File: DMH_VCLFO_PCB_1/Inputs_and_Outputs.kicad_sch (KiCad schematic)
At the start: 7 parts, among them J1 TS_Jack_6.35mm_Sw, J2 TS_Jack_6.35mm_Sw, J200 IDC_02x05, J3 TS_Jack_6.35mm_Sw, J5 TS_Jack_6.35mm_Sw, J50 Conn_01x06, J60 Conn_01x06

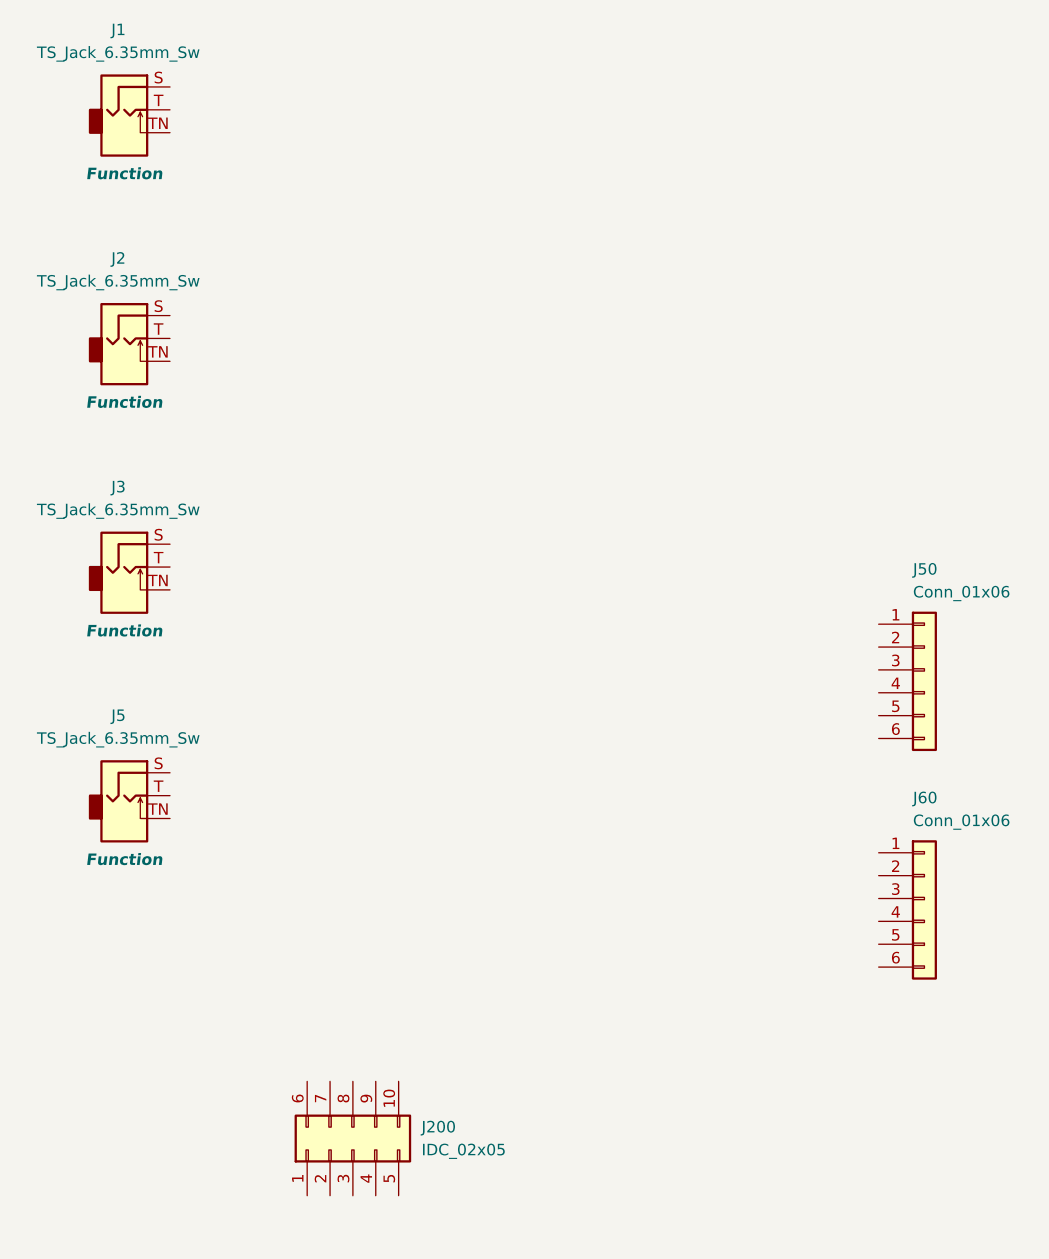
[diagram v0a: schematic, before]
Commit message: schematic design in progress
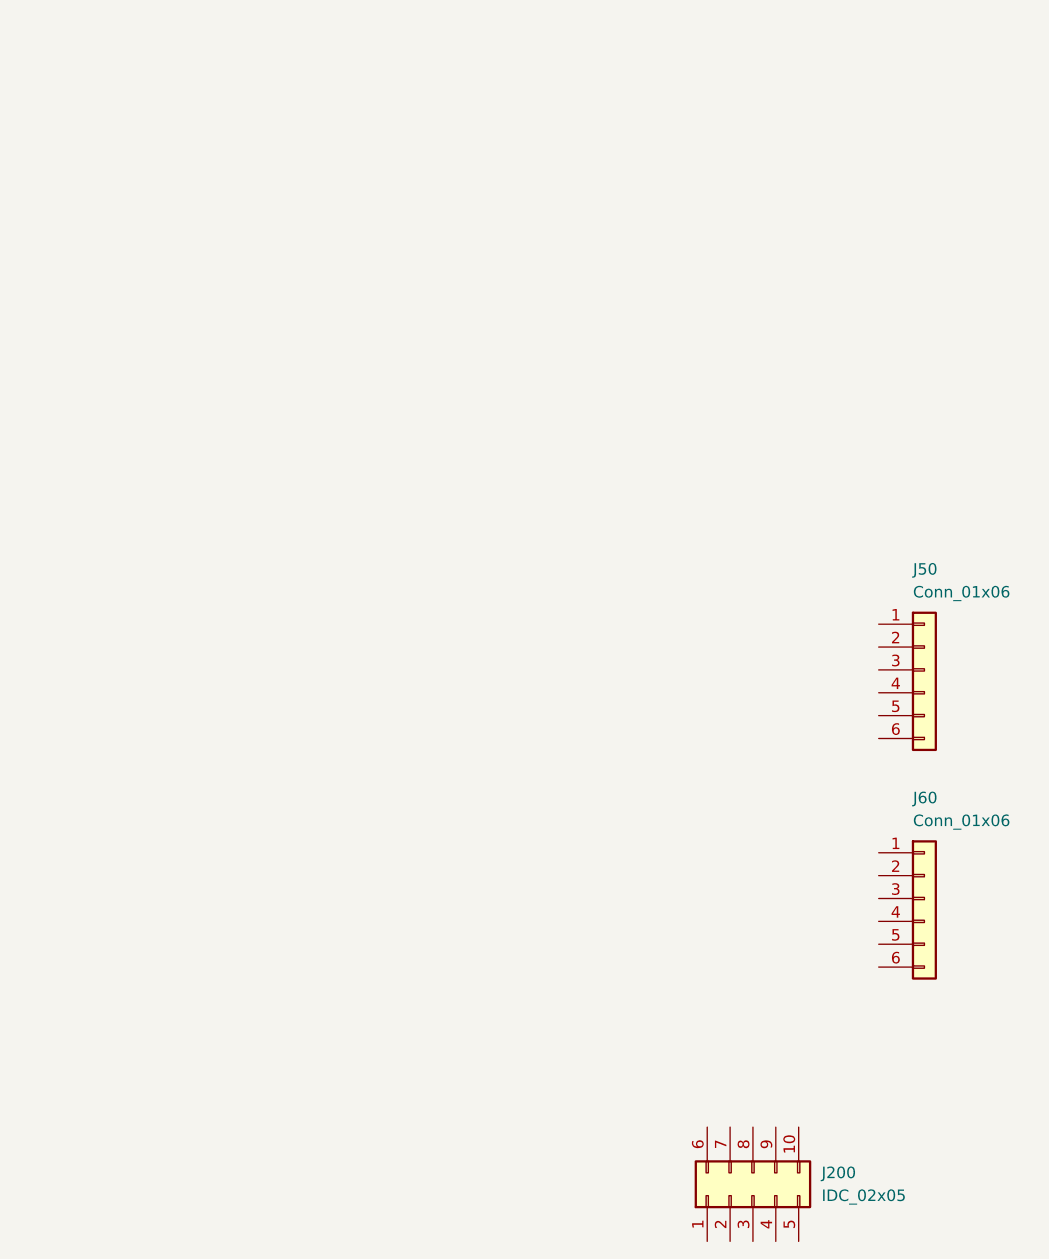
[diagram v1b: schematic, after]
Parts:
- removed J1, J2, J3, J5: TS_Jack_6.35mm_Sw, SynthStuff:CUI_MJ-63052A, symbol SynthStuff:TS_Jack_6.35mm_Sw
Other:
- moved on the sheet: J200

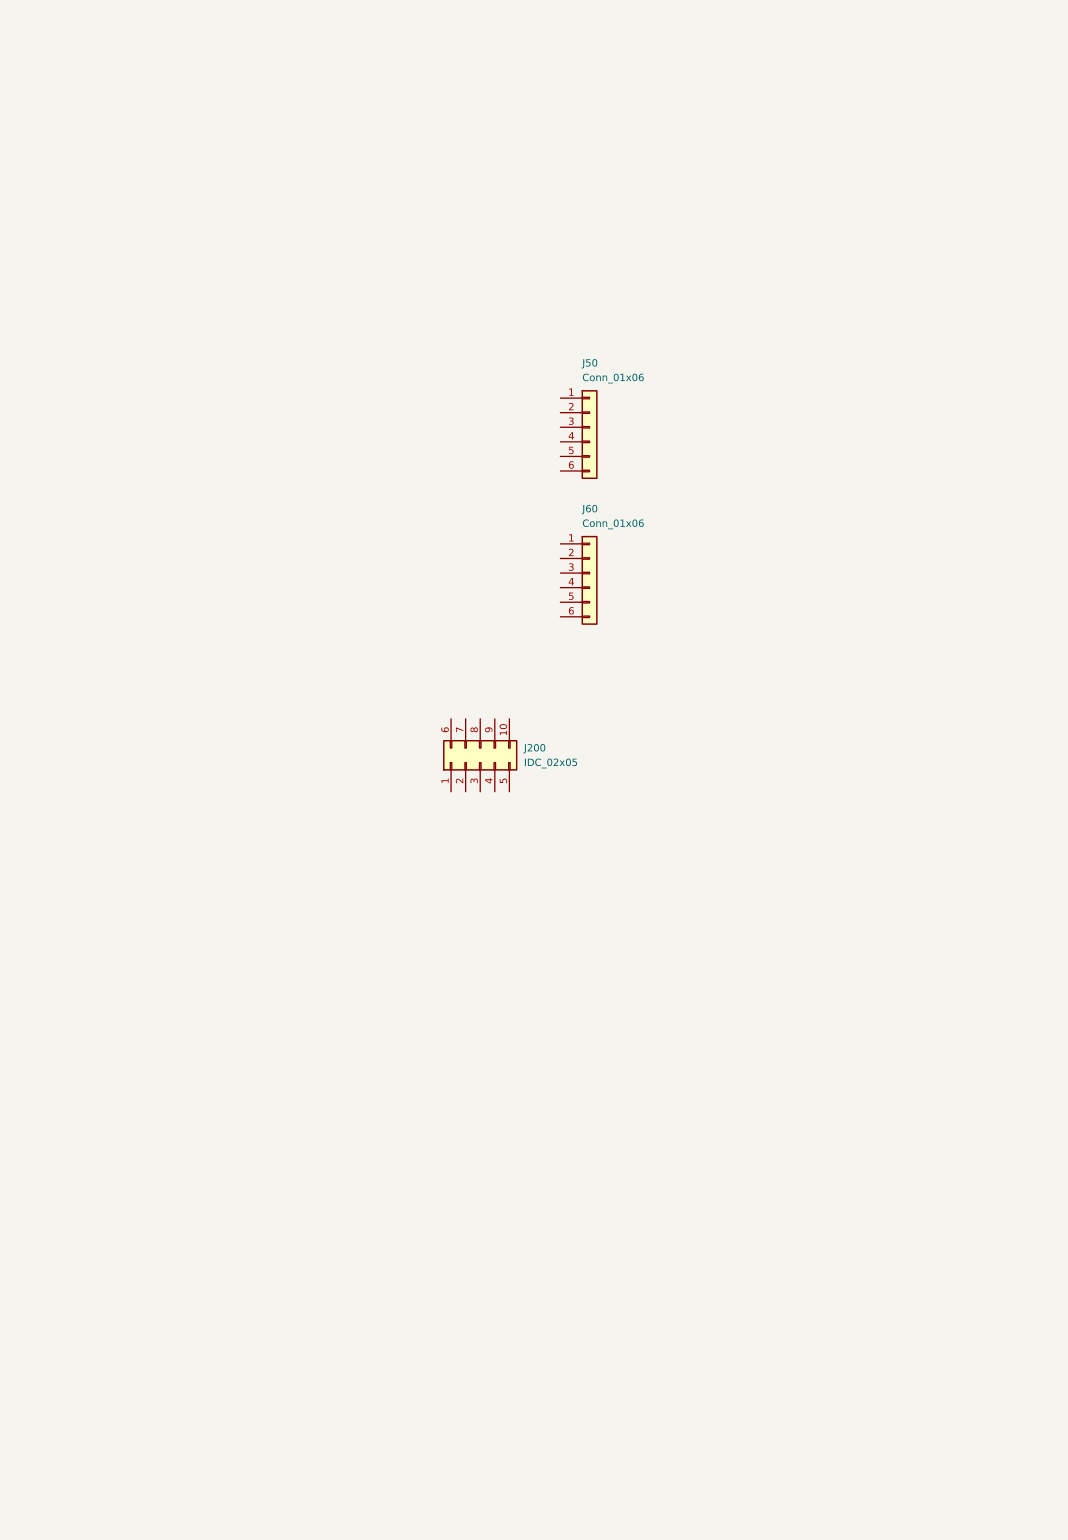
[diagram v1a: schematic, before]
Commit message: Ready for breadboarding
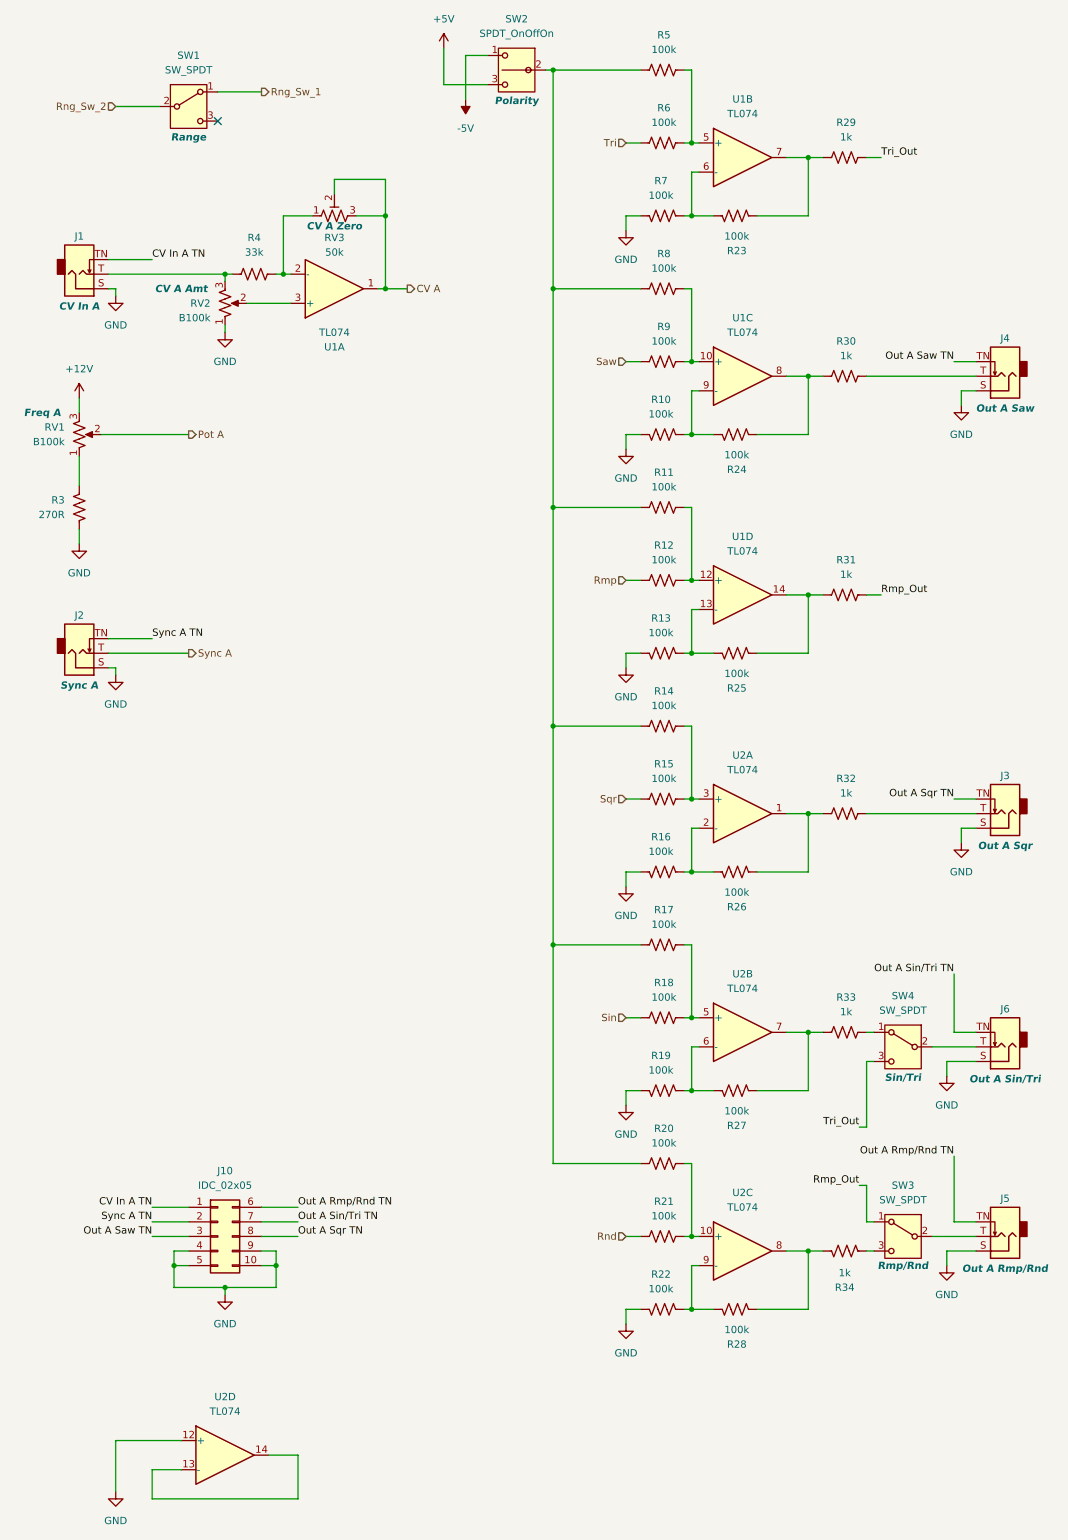
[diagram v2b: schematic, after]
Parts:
- removed J200: IDC_02x05, SynthStuff:IDC-Header_2x05_P2.54mm_Vertical_BackBone, symbol SynthStuff:BackBone_Connector_10Pin
- removed J50, J60: Conn_01x06, Connector_PinSocket_2.54mm:PinSocket_1x06_P2.54mm_Vertical, symbol Connector_Generic:Conn_01x06
- added J1, J2, J3, J4, J5, J6: TS_Jack_6.35mm_Sw, SynthStuff:CUI_MJ-63052A, symbol SynthStuff:TS_Jack_6.35mm_Sw
- added J10: IDC_02x05, SynthStuff:IDC-Header_2x05_P2.54mm_Vertical_BackBone, symbol SynthStuff:BackBone_Connector_10Pin
- added R10, R11, R12, R13, R14, R15, R16, R17, R18, R19, R20, R21, R22, R23, R24, R25, R26, R27, R28, R5, R6, R7, R8, R9: 100k, Resistor_THT:R_Axial_DIN0207_L6.3mm_D2.5mm_P7.62mm_Horizontal, symbol Device:R_US
- added R29, R30, R31, R32, R33, R34: 1k, Resistor_THT:R_Axial_DIN0207_L6.3mm_D2.5mm_P7.62mm_Horizontal, symbol Device:R_US
- added R3: 270R, Resistor_THT:R_Axial_DIN0207_L6.3mm_D2.5mm_P7.62mm_Horizontal, symbol Device:R_US
- added R4: 33k, Resistor_THT:R_Axial_DIN0207_L6.3mm_D2.5mm_P7.62mm_Horizontal, symbol Device:R_US
- added RV1, RV2: B100k, SynthStuff:Potentiometer_TT_P110KH1, symbol Device:R_Potentiometer_US
- added RV3: 50k, Potentiometer_THT:Potentiometer_Bourns_3296X_Horizontal, symbol Device:R_Potentiometer_Trim_US
- added SW1, SW3, SW4: SW_SPDT, SynthStuff:Toggle_Switch_TE, symbol Switch:SW_SPDT
- added SW2: SPDT_OnOffOn, SynthStuff:Toggle_Switch_TE, symbol SynthStuff:SW_SPDT_OnOffOn
- added U1, U2: TL074, Package_DIP:DIP-14_W7.62mm_Socket, symbol Amplifier_Operational:TL074
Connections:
- new net: R24.2, R30.1, U1.8
- new net: J4.T, R30.2
- new net: R26.2, R32.1, U2.1
- new net: R16.1, R26.1, U2.2 (-)
- new net: R14.2, R15.2, U2.3 (+)
- new net: J5.T, SW3.2 (B)
- new net: R34.1, SW3.3 (C)
- new net: R22.1, R28.1, U2.9 (-)
- new net: R4.2, RV3.1, U1.2 (-)
- new net: R11.1, R14.1, R17.1, R20.1, R5.1, R8.1, SW2.2 (B)
- new net: R5.2, R6.2, U1.5 (+)
- new net: R25.2, R31.1, U1.14
- new net: R20.2, R21.2, U2.10 (+)
- new net: J1.T, R4.1, RV2.3
- new net: R8.2, R9.2, U1.10 (+)
- new net: R3.1, RV1.1
- new net: R19.1, R27.1, U2.6 (-)
- new net: R11.2, R12.2, U1.12 (+)
- new net: R13.1, R25.1, U1.13 (-)
- new net: R28.2, R34.2, U2.8
- new net: R17.2, R18.2, U2.5 (+)
- new net: RV2.2, U1.3 (+)
- new net: R27.2, R33.1, U2.7
- new net: R33.2, SW4.1 (A)
- new net: R23.2, R29.1, U1.7
- new net: R10.1, R24.1, U1.9 (-)
- new net: J6.T, SW4.2 (B)
- new net: R23.1, R7.1, U1.6 (-)
- new net: J3.T, R32.2
- new net: U2.13 (-), U2.14
- new net +12V: RV1.3
- new net +5V: SW2.3 (C)
- new net -5V: SW2.1 (A)
- new net CV A: RV3.2, RV3.3, U1.1
- new net CV In A TN: J1.TN, J10.1 (Pin_1)
- new net GND: J1.S, J10.10 (Pin_10), J10.4 (Pin_4), J10.5 (Pin_5), J10.9 (Pin_9), J2.S, J3.S, J4.S, J5.S, J6.S, R10.2, R13.2, R16.2, R19.2, R22.2, R3.2, R7.2, RV2.1, U2.12 (+)
- new net Out A Rmp/Rnd TN: J10.6 (Pin_6), J5.TN
- new net Out A Saw TN: J10.3 (Pin_3), J4.TN
- new net Out A Sin/Tri TN: J10.7 (Pin_7), J6.TN
- new net Out A Sqr TN: J10.8 (Pin_8), J3.TN
- new net Pot A: RV1.2
- new net Rmp: R12.1
- new net Rmp_Out: R31.2, SW3.1 (A)
- new net Rnd: R21.1
- new net Rng_Sw_1: SW1.1 (A)
- new net Rng_Sw_2: SW1.2 (B)
- new net Saw: R9.1
- new net Sin: R18.1
- new net Sqr: R15.1
- new net Sync A: J2.T
- new net Sync A TN: J10.2 (Pin_2), J2.TN
- new net Tri: R6.1
- new net Tri_Out: R29.2, SW4.3 (C)
- no-connect marks 0 -> 1
